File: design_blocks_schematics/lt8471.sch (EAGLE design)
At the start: 24 parts, among them IC2 LT8471EFE#PBF

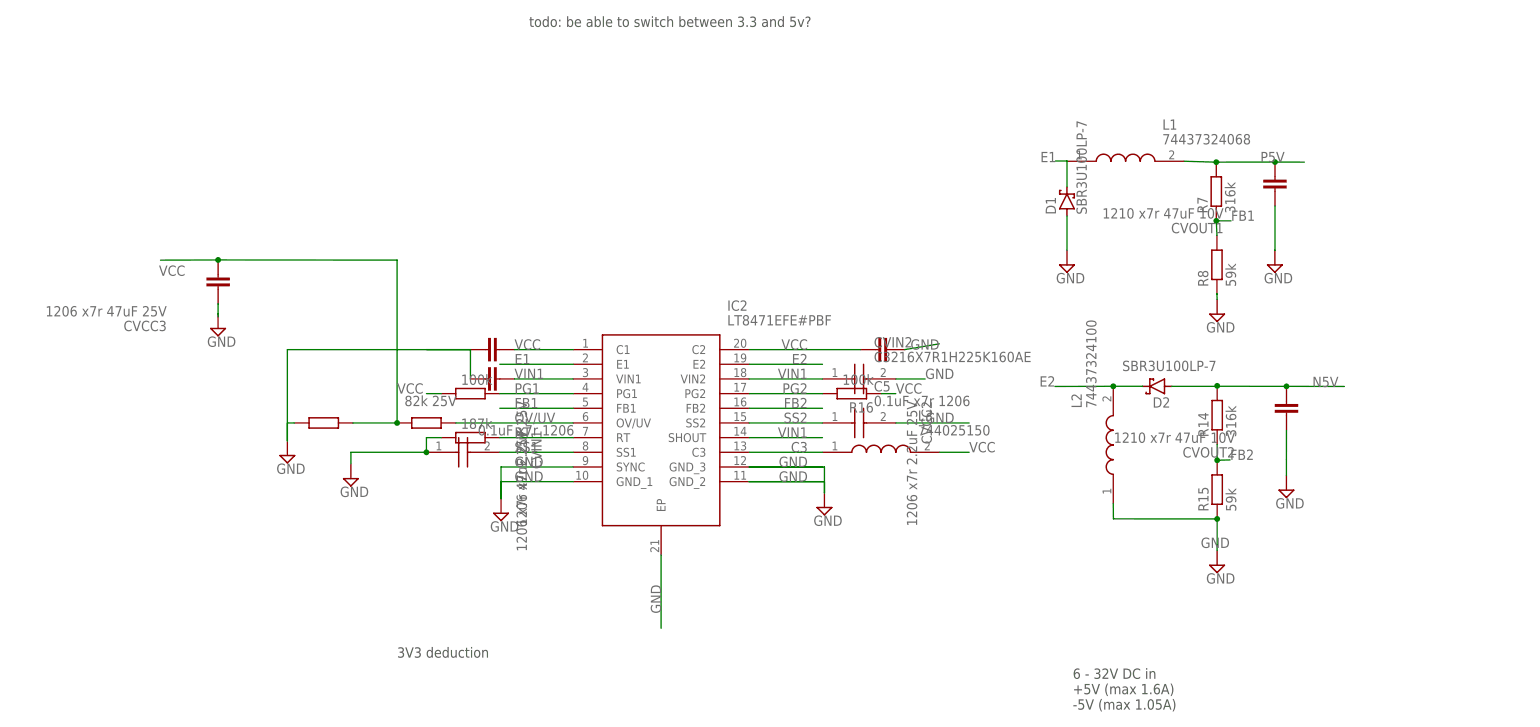
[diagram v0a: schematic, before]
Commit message: cleanup schematic/WIP layout
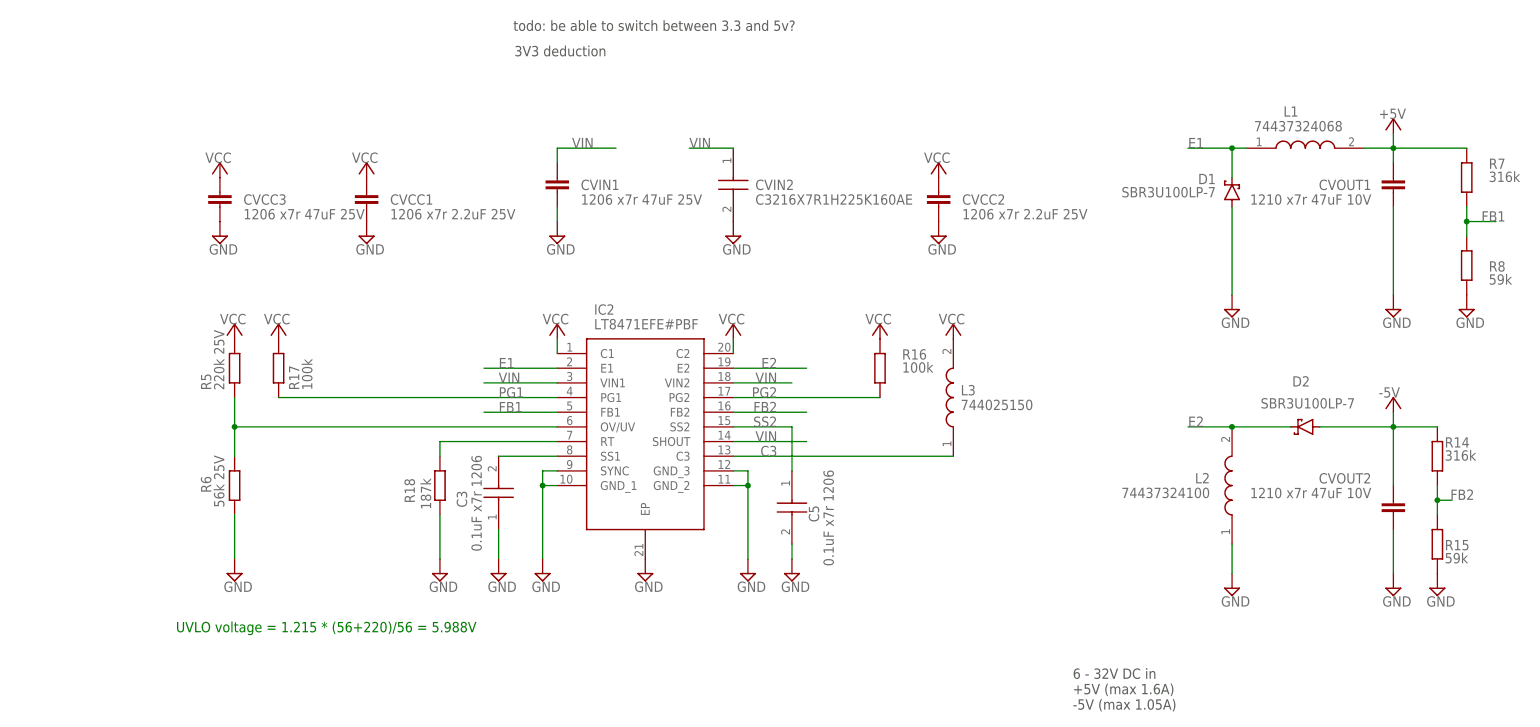
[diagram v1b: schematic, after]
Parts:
- R5: value 261k 25V -> 220k 25V
- R6: value 82k 25V -> 56k 25V
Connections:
- net N5V renamed -5V
- net P5V renamed +5V
- net RT renamed N$1
- net VIN1 renamed VIN
- removed net OV/UV: IC2.OV/UV, R5.2
- new net N$4: IC2.OV/UV, R5.1, R6.2
- net VCC: now also R5.2; no longer R5.1, R6.2
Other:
- note added: "UVLO voltage = 1.215 * (56+220)/56 = 5.988V"
- moved on the sheet: C5, CVCC2, CVCC3, CVIN1, CVIN2, CVOUT1, CVOUT2, D1, D2, IC2, L1, L2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
